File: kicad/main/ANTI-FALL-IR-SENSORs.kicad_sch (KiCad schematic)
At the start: 11 parts, among them Q5 2302V, Q6 2302V

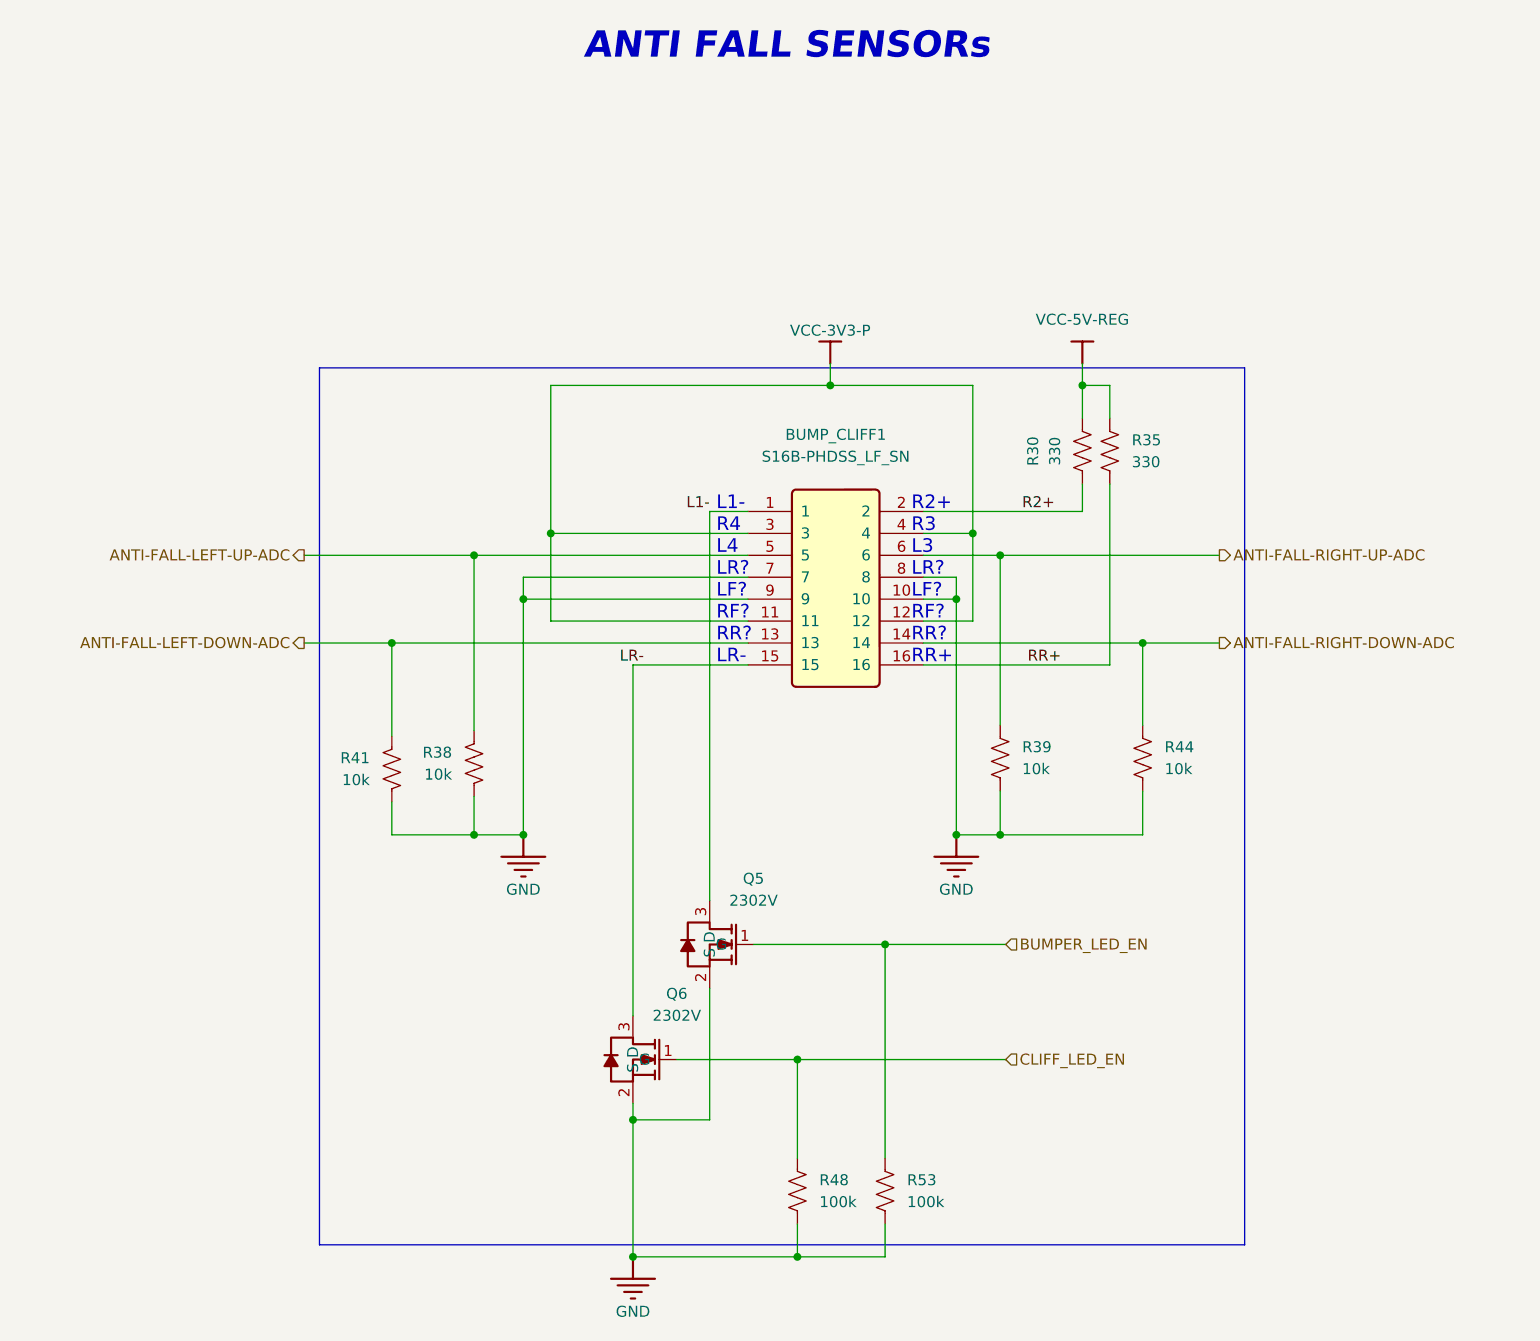
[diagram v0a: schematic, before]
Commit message: Second review round
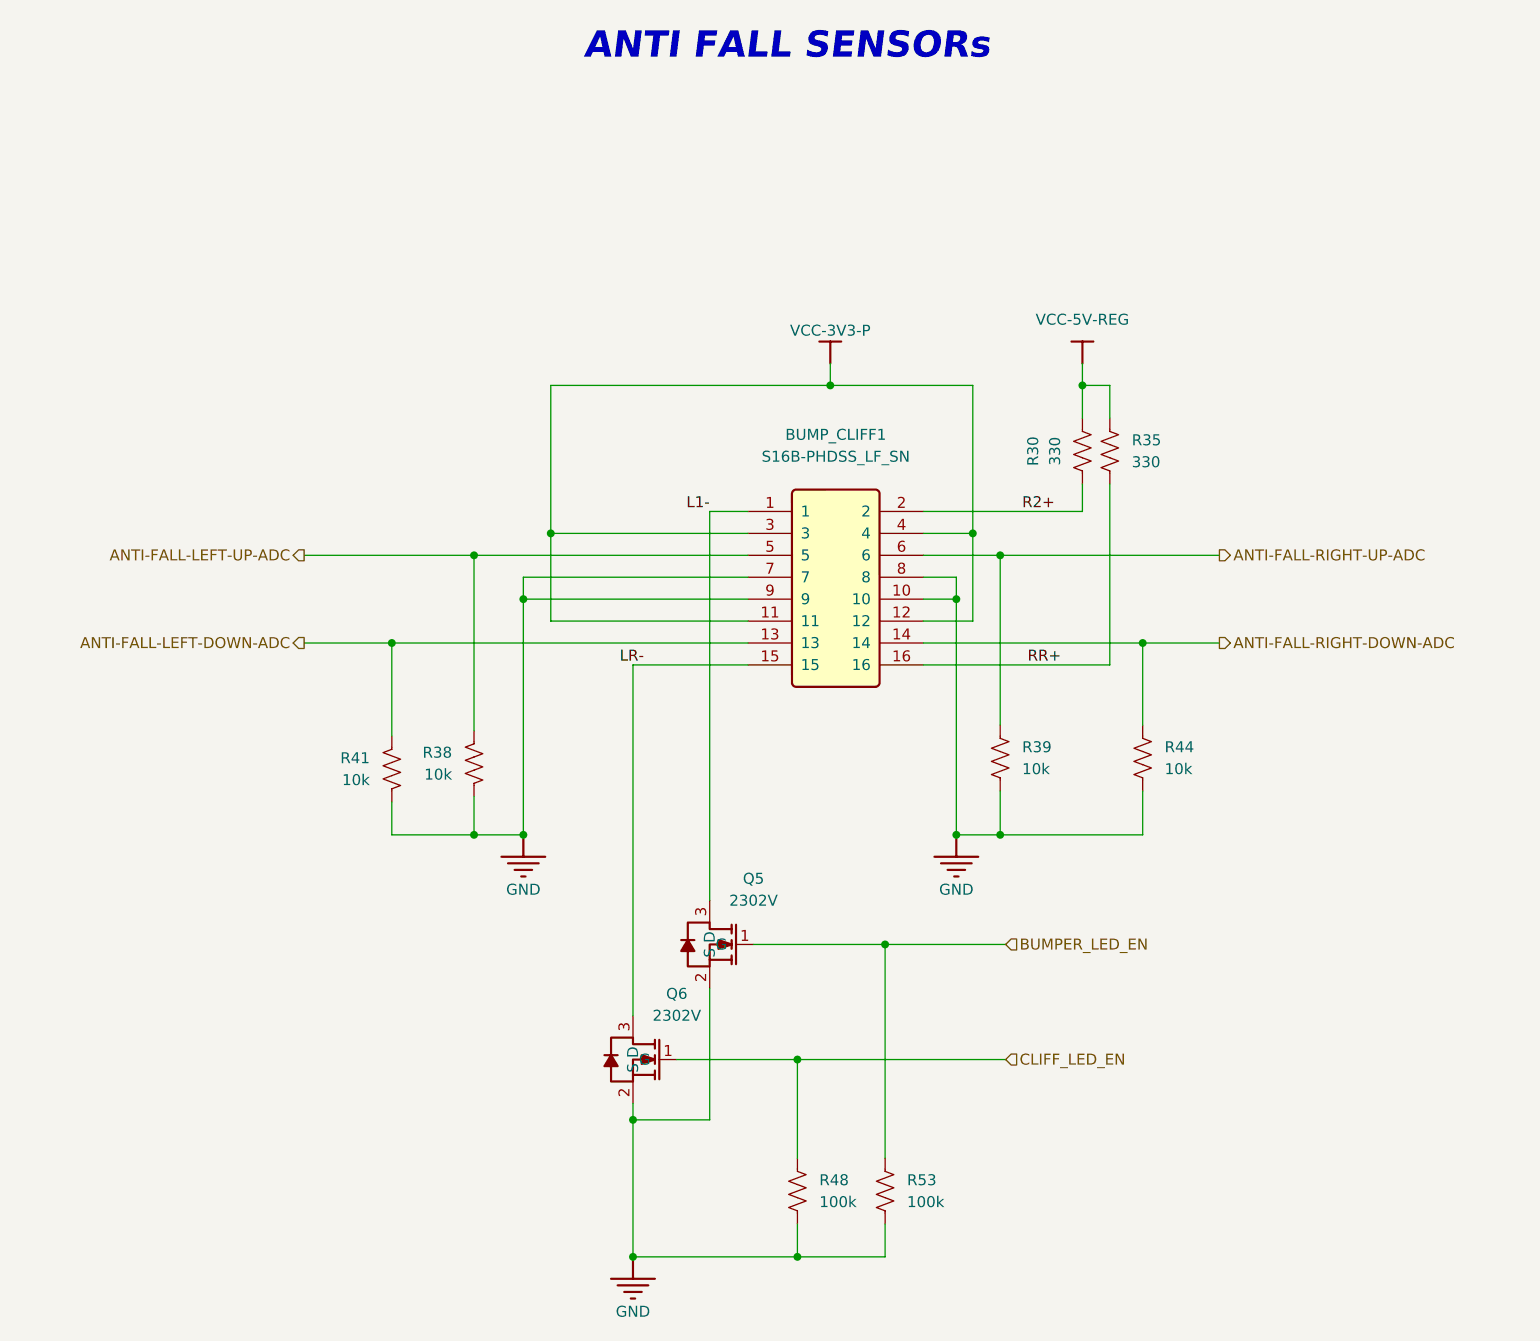
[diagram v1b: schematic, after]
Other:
- note removed: "L1- R4 L4 LR? LF? RF? RR? LR-"
- note removed: "R2+ R3 L3 LR? LF? RF? RR? RR+"
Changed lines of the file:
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@@
 	(generator_version "10.0")
 	(paper "A2")
-	(rectangle
-		(start 244.348 178.308)
-		(end 351.536 279.908)
-		(stroke
-			(width 0)
-			(type solid)
-		)
-		(fill
-			(type color)
-			(color 72 0 0 1)
-		)
-	)
-	(text "L1-\nR4\nL4\nLR?\nLF?\nRF?\nRR?\nLR-"
-		(exclude_from_sim no)
-		(at 290.322 202.946 0)
-		(effects
-			(font
-				(size 1.5748 1.5748)
-			)
-			(justify left)
-		)
-	)
 	(text "ANTI FALL SENSORs"
 		(exclude_from_sim no)
@@
 		)
 	)
-	(text "R2+\nR3\nL3\nLR?\nLF?\nRF?\nRR?\nRR+"
-		(exclude_from_sim no)
-		(at 312.928 202.946 0)
-		(effects
-			(font
-				(size 1.5748 1.5748)
-			)
-			(justify left)
-		)
-	)
